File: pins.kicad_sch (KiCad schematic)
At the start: 10 parts, among them J2 AXK640347YG, J3 Conn_01x09, J6 Conn_01x40_Pin

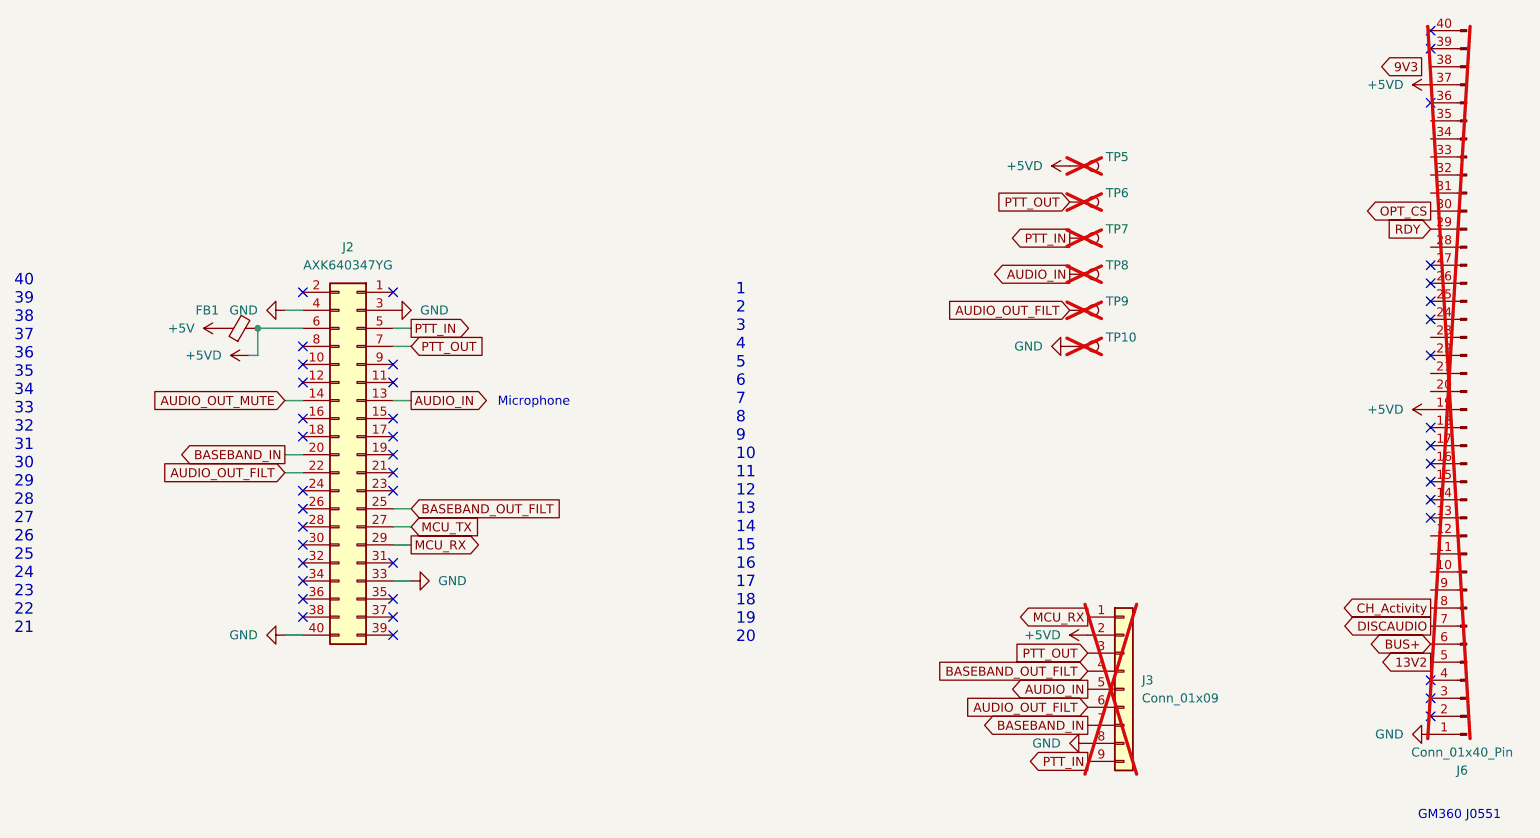
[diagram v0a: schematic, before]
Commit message: V1.0 Final touch
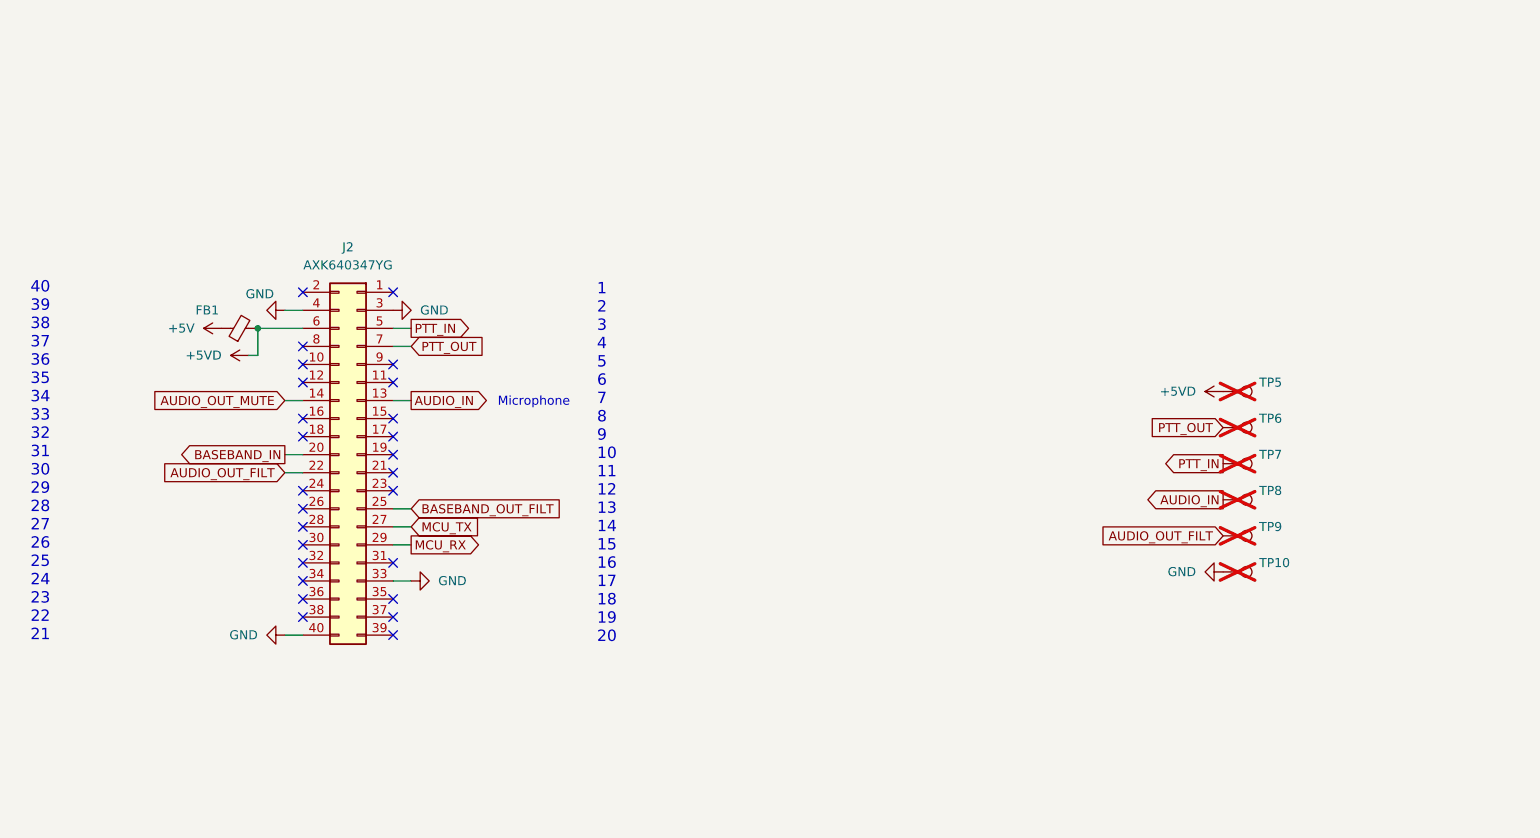
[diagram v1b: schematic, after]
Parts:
- removed J3: Conn_01x09, Connector_PinSocket_2.00mm:PinSocket_1x09_P2.00mm_Horizontal, symbol Connector_Generic:Conn_01x09
- removed J6: Conn_01x40_Pin, Connector_FFC-FPC:Hirose_FH12-40S-0.5SH_1x40-1MP_P0.50mm_Horizontal, symbol Connector:Conn_01x40_Pin
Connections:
- no-connect marks 43 -> 26
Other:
- note removed: "GM360 J0551"
- moved on the sheet: TP10, TP5, TP6, TP7, TP8, TP9
